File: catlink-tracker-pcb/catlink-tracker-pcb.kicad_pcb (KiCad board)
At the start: 4 copper layers, 17.6 x 35.1 mm, 34 parts, among them J1 S2B-PH-K, J2 U.FL, U1 STM32L412K8Tx, U2 TLV75530PDBV, U3 Ai-Thinker-Ra-01S, U4 E108-GN03

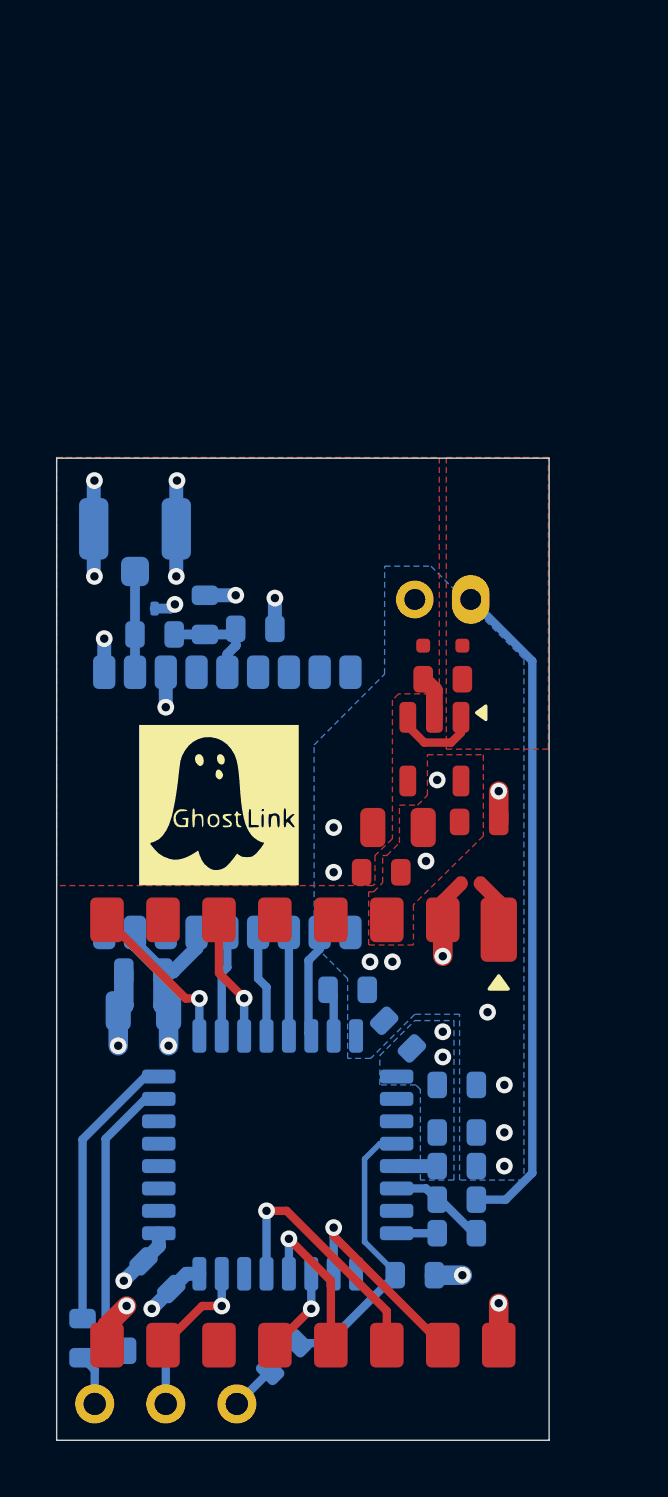
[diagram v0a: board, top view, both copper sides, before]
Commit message: v0.1
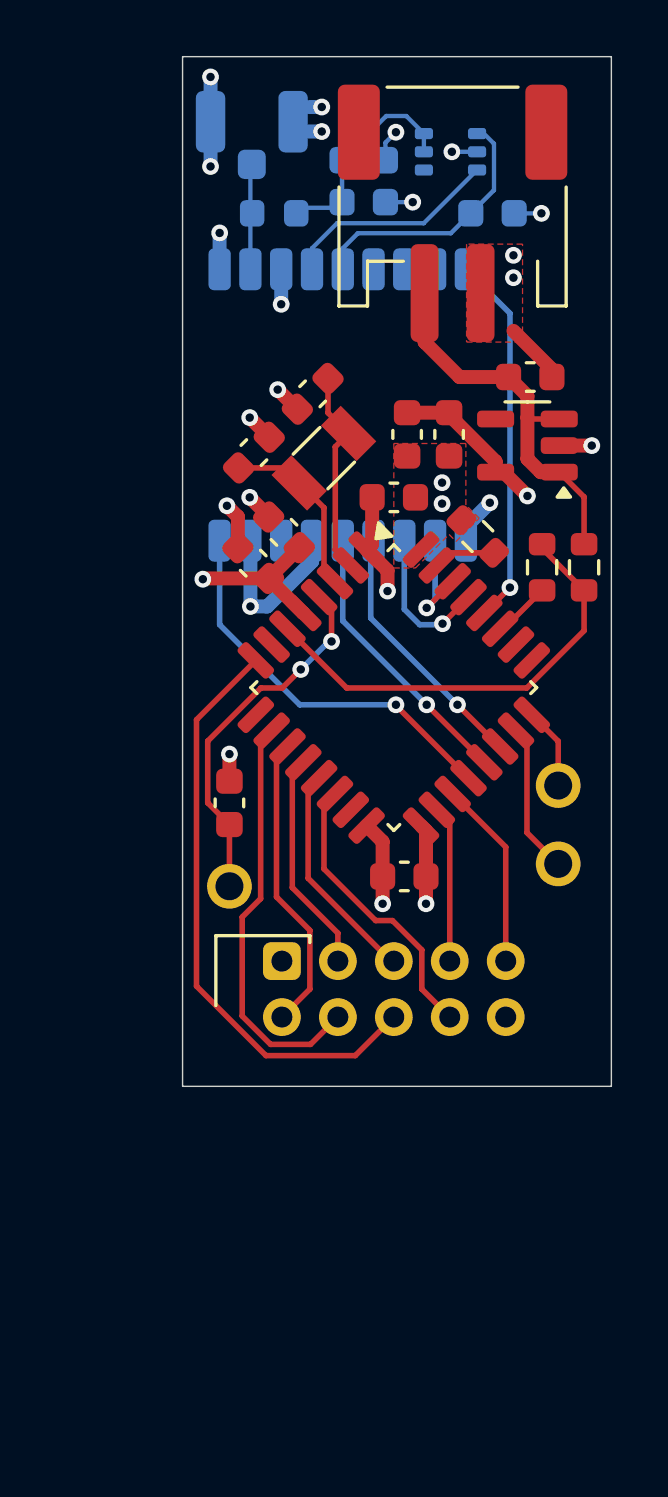
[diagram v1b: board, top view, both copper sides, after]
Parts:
- removed C14: 100p, Custom:C_0603_1608Metric
- removed D1: ESD5Z6.0T1G, Custom:D_SOD-523
- removed D2, D3: TPD1E0B04DPY, Custom:D_Texas_DPY0002A_0.6x1mm_P0.65mm
- removed R4: 10k, Custom:R_0603_1608Metric
- removed R5, R6: 100r, Custom:R_0603_1608Metric
- added J3: U.FL, Connector_Coaxial:U.FL_Hirose_U.FL-R-SMT-1_Vertical, B.Cu at (120.8, 80.5)
- added Y1: ABS07-32.768KHZ, Crystal:Crystal_SMD_3215-2Pin_3.2x1.5mm, F.Cu at (123.3, 92.1)
- C1, C2, C3, C4, C5, C6: footprint Custom:C_0603_1608Metric -> Capacitor_SMD:C_0603_1608Metric; moved to F.Cu
- C10, C12: value 100n -> 1u; footprint Custom:C_0603_1608Metric -> Capacitor_SMD:C_0603_1608Metric
- C11, C9: value 10u -> 1u; footprint Custom:C_0805_2012Metric -> Capacitor_SMD:C_0603_1608Metric
- C13: value 100n -> 10n; footprint Custom:C_0603_1608Metric -> Capacitor_SMD:C_0603_1608Metric
- C7, C8: value 1u -> 18p; footprint Custom:C_0603_1608Metric -> Capacitor_SMD:C_0603_1608Metric
- G***: moved to B.Cu
- J1: value S2B-PH-K -> S2B-PH-SM4; footprint Connector_JST:JST_PH_S2B-PH-K_1x02_P2.00mm_Horizontal -> Connector_JST:JST_PH_S2B-PH-SM4-TB_1x02-1MP_P2.00mm_Horizontal; moved to F.Cu
- J2: value U.FL -> S10B-PHDSS; footprint Connector_Coaxial:U.FL_Hirose_U.FL-R-SMT-1_Vertical -> Connector_JST:JST_PHD_S10B-PHDSS_2x05_P2.00mm_Horizontal; moved to F.Cu
- L1: value 82n -> 68nH; footprint Custom:L_0603_1608Metric -> Inductor_SMD:L_0603_1608Metric
- R1, R2, R3: footprint Custom:R_0603_1608Metric -> Resistor_SMD:R_0603_1608Metric; moved to F.Cu
- TP1, TP2, TP3: value TestPoint -> ~; footprint Custom:TestPoint_THT_D1.4mm_Drill0.8mm -> Custom:TestPoint; moved to F.Cu
- U1: footprint Custom:LQFP-32_7x7mm_P0.8mm -> Package_QFP:LQFP-32_7x7mm_P0.8mm; moved to F.Cu
- U2: footprint Custom:SOT-23-5 -> Package_TO_SOT_SMD:SOT-23-5
- U3: value Ai-Thinker-Ra-01S -> E108-GN03; footprint Custom:Ai-Thinker-Ra-01S -> Custom:E108-GN03; moved to B.Cu
- U4: value E108-GN03 -> TPS22919DCKR; footprint Custom:E108-GN03 -> Package_TO_SOT_SMD:SOT-363_SC-70-6
- moved C11 31.1 mm to (129.4, 83.3), turned to 0 degrees
- moved C12 30.1 mm to (124.8, 81.5), turned to 0 degrees
- moved TP3 27.6 mm to (131.7, 103.8)
- moved U3 26.0 mm to (124.0, 90.2), turned to 90 degrees
- moved U4 24.6 mm to (127.9, 81.2), turned to 180 degrees
- moved R3 24.0 mm to (131.2, 96.0), turned to 90 degrees
- moved TP2 23.9 mm to (131.7, 106.6)
- moved C1 23.3 mm to (126.3, 91.2), turned to -90 degrees
- moved R2 23.1 mm to (132.7, 96.0), turned to 90 degrees
- moved C4 22.7 mm to (120.8, 95.8), turned to 135 degrees
- moved C5 22.3 mm to (121.9, 94.8), turned to 135 degrees
- moved C2 19.2 mm to (125.8, 93.5), turned to 0 degrees
- moved TP1 18.5 mm to (120.0, 107.4)
- moved C6 18.1 mm to (120.0, 104.4), turned to -90 degrees
- moved U1 17.2 mm to (125.8, 100.3), turned to -45 degrees
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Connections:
- C1 pad 1: +3V0 -> +3.0V
- C10 pad 1: +3V0 -> +3.0V
- C11 pad 1: +3V0 -> /GNSS_VCC_RF
- C12 pad 1: +3V0 -> Net-(U4-QOD)
- C13 pad 1: /VCC_RF -> Net-(U4-QOD)
- C2 pad 1: +3V0 -> +3.0V
- C3 pad 1: +3V0 -> +3.0V
- C4 pad 1: +3V0 -> +3.0V
- C5 pad 1: +3V0 -> +3.0V
- C6 pad 1: Net-(U1-NRST) -> GND
- C6 pad 2: GND -> /NRST
- C7 pad 1: /VIN -> GND
- C7 pad 2: GND -> /OSC32_IN
- C8 pad 1: +3V0 -> GND
- C8 pad 2: GND -> /OSC32_OUT
- C9 pad 1: +3V0 -> /V_{IN}
- J1 pad 2: /VIN -> /V_{IN}
- J2 pad 1: /RF_IN -> GND
- J2 pad 2: GND -> /SX126x_SCK
- L1 pad 1: /RF_IN -> /GNSS_RF_IN
- L1 pad 2: /VCC_RF -> Net-(U4-QOD)
- R1 pad 1: /BOOT0 -> GND
- R1 pad 2: GND -> /BOOT0
- R2 pad 1: /VIN -> /VIN_ADC
- R2 pad 2: /VIN_ADC -> /V_{IN}
- R3 pad 1: /VIN_ADC -> /VIN_ADC_DIV_EN
- R3 pad 2: /VIN_ADC_DIV_EN -> /VIN_ADC
- TP1 pad 1: /~{NRST} -> /NRST
- U1 pad 1: +3V0 -> +3.0V
- U1 pad 10: /~{NSS} -> /SX126x_BUSY
- U1 pad 11: /SCK -> /SX126x_SCK
- U1 pad 12: /MISO -> /SX126x_MISO
- U1 pad 13: /MOSI -> /SX126x_MOSI
- U1 pad 14: unconnected-(U1-PB0-Pad14) -> /SX126x_NSS
- U1 pad 15: /BUSY -> unconnected-(U1-PB1-Pad15)
- U1 pad 17: +3V0 -> +3.0V
- U1 pad 18: unconnected-(U1-PA8-Pad18) -> /SX126x_REST
- U1 pad 19: unconnected-(U1-PA9-Pad19) -> /SX126x_DIO3
- U1 pad 2: unconnected-(U1-PC14-Pad2) -> /OSC32_IN
- U1 pad 20: unconnected-(U1-PA10-Pad20) -> /GNSS_RESET_N
- U1 pad 21: unconnected-(U1-PA11-Pad21) -> /GNSS_ON_OFF
- U1 pad 22: unconnected-(U1-PA12-Pad22) -> /GNSS_1PPS
- U1 pad 23: Net-(U1-PA13) -> /SWDIO
- U1 pad 24: Net-(U1-PA14) -> /SWCLK
- U1 pad 25: /DIO3 -> unconnected-(U1-PA15-Pad25)
- U1 pad 26: /ON_OFF -> unconnected-(U1-PB3-Pad26)
- U1 pad 27: /DIO1 -> /VIN_ADC_DIV_EN
- U1 pad 28: /1PPS -> /GNSS_MODEL_SET
- U1 pad 3: unconnected-(U1-PC15-Pad3) -> /OSC32_OUT
- U1 pad 4: Net-(U1-NRST) -> /NRST
- U1 pad 5: +3V0 -> +3.0V
- U1 pad 8: /VIN_ADC_DIV_EN -> /SX126x_DIO1
- U2 pad 1: /VIN -> /V_{IN}
- U2 pad 3: /VIN -> /V_{IN}
- U2 pad 5: +3V0 -> +3.0V
- U3 pad 1: /LoRa_ANT -> GND
- U3 pad 10: /BUSY -> GND
- U3 pad 11: unconnected-(U3-RXEN-Pad11) -> /GNSS_RF_IN
- U3 pad 12: /SCK -> GND
- U3 pad 13: /MISO -> /GNSS_ANT_ON
- U3 pad 14: /MOSI -> /GNSS_VCC_RF
- U3 pad 15: /~{NSS} -> unconnected-(U3-NC-Pad15)
- U3 pad 16: GND -> unconnected-(U3-NC-Pad16)
- U3 pad 2: GND -> /GNSS_TXD
- U3 pad 3: +3V0 -> /GNSS_RxD
- U3 pad 4: unconnected-(U3-~{RESET}-Pad4) -> /GNSS_1PPS
- U3 pad 5: unconnected-(U3-TXEN-Pad5) -> /GNSS_ON_OFF
- U3 pad 6: /DIO1 -> +3.0V
- U3 pad 8: /DIO3 -> +3.0V
- U3 pad 9: GND -> /GNSS_RESET_N
- U4 pad 1: GND -> /GNSS_VCC_RF
- U4 pad 2: /GNSS_TXD -> GND
- U4 pad 3: /GNSS_RxD -> /GNSS_ANT_ON
- U4 pad 4: /1PPS -> unconnected-(U4-NC-Pad4)
- U4 pad 5: /ON_OFF -> Net-(U4-QOD)
- U4 pad 6: +3V0 -> Net-(U4-QOD)
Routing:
- net /VIN: track 27.0 -> 0.00 mm
- net +3.0V: track 0.00 -> 24.0 mm, vias 0 -> 5
- net /SX126x_DIO1: track 0.00 -> 21.2 mm
- net /SX126x_BUSY: track 0.00 -> 14.9 mm
- net /GNSS_RESET_N: track 0.00 -> 14.2 mm, vias 0 -> 1
- net /V_{IN}: track 0.00 -> 13.9 mm
- net /GNSS_MODEL_SET: track 0.00 -> 13.3 mm, vias 0 -> 1
- net /NRST: track 0.00 -> 13.2 mm, vias 0 -> 2
- net /VIN_ADC: track 3.51 -> 16.0 mm
- net /SX126x_SCK: track 0.00 -> 10.7 mm
- net Net-(U1-NRST): track 10.5 -> 0.00 mm
- net Net-(U1-PA13): track 10.4 -> 0.00 mm
- net /SX126x_NSS: track 0.00 -> 10.4 mm
- net +3V0: track 10.3 -> 0.00 mm, vias 6 -> 0
- net Net-(U1-PA14): track 10.1 -> 0.00 mm
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- added copper zone on In1.Cu, net +3.0V
- removed copper zone on B.Cu, net +3V0
- removed copper zone on F.Cu, net +3V0
- removed copper zone on In1.Cu, net +3V0
- removed copper zone on F.Cu, net /VIN
- removed copper zone on B.Cu, net GND
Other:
- board size 17.6 x 35.1 mm -> 15.3 x 36.8 mm
- board text removed: "3-5.5V"
